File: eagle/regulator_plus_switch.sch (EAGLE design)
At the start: 60 parts, among them IC1 LT1352PA, IC2 LT1352PA, IC3 DG419DJN, IC4 LT1352PA, T1 2N3904, T2 2N3904

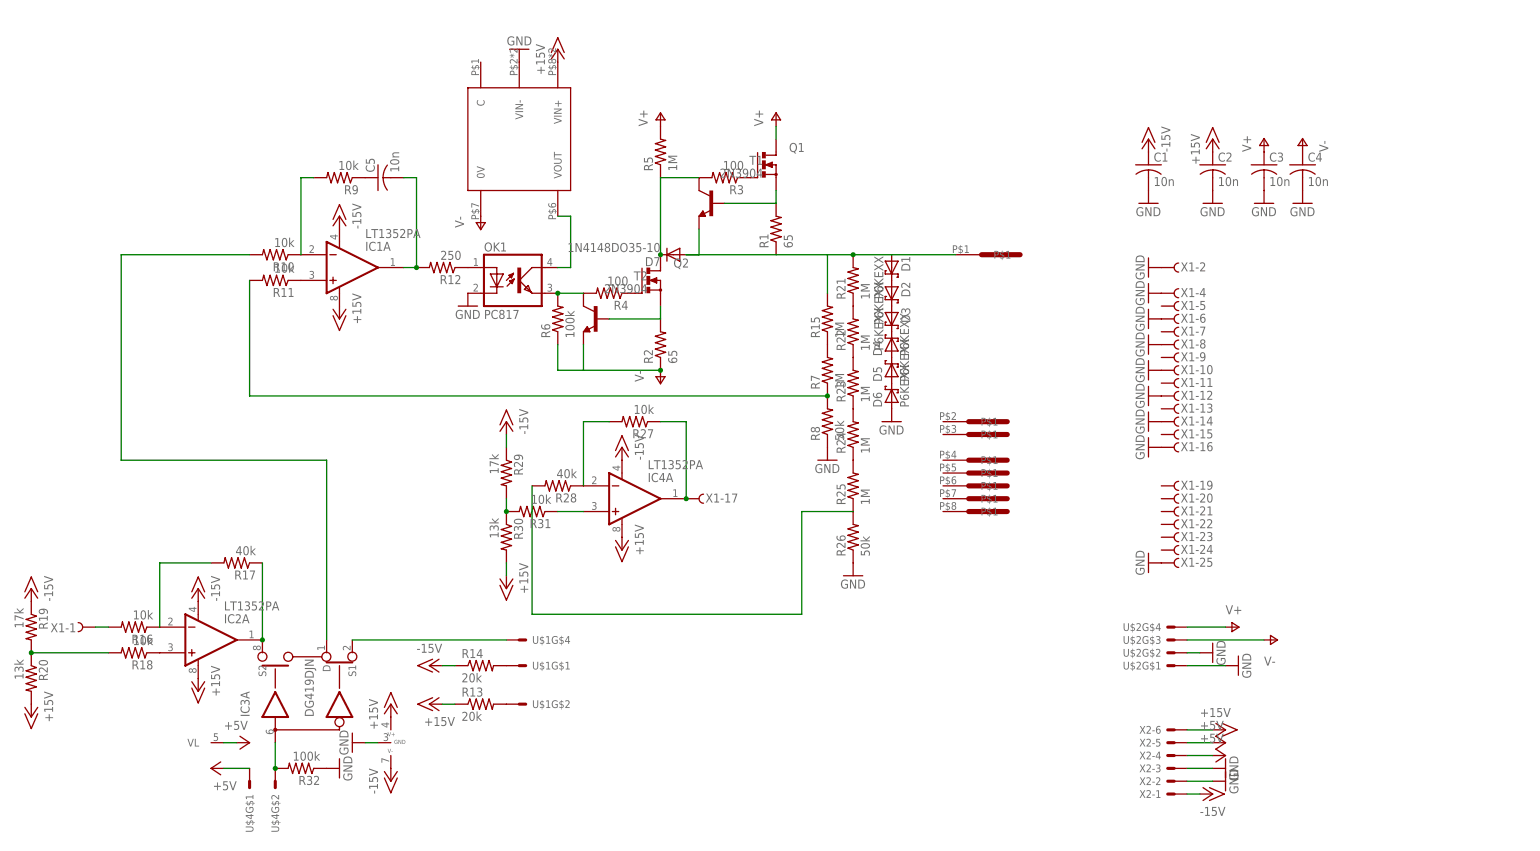
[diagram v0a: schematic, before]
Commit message: pa 97 circuit
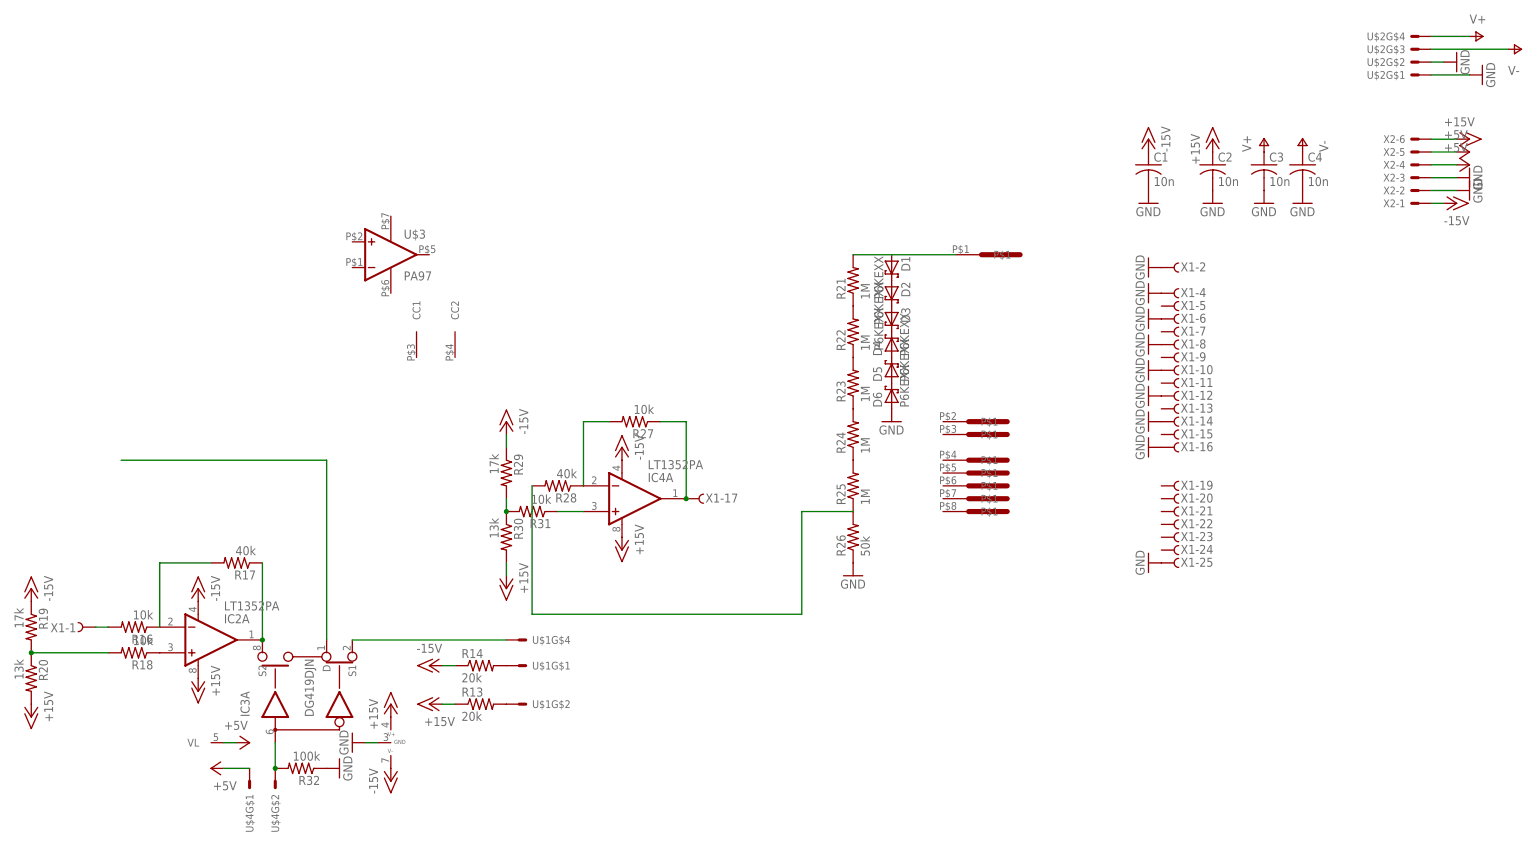
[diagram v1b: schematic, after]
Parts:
- removed C5: 10n, rcl:C-US075-032X103
- removed D7: 1N4148DO35-10, diode:1N4148DO35-10
- removed DC1: (no value), dc-dc-converter:NCS
- removed IC1: LT1352PA, linear-technology:LT1352PA
- removed OK1: PC817, optocoupler:PC817
- removed Q1, Q2: (no value), transistor-power:PMOSFET_NTO220BV
- removed R1, R2: 65, rcl:R-US_0207/10
- removed R10, R11, R9: 10k, rcl:R-US_0207/10
- removed R12: 250, rcl:R-US_0207/15
- removed R15, R5, R7: 1M, resistor:R-US_0414/15
- removed R3, R4: 100, rcl:R-US_0207/10
- removed R6: 100k, rcl:R-US_0207/10
- removed R8: 50k, rcl:R-US_0207/10
- removed T1, T2: 2N3904, transistor:2N3904
- added U$3: PA97, apex:PA97
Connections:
- removed net N$11: Q2.G, R4.1
- removed net N$12: OK1.EMIT, R4.2, R6.2, T2.C
- removed net N$14: Q2.S, R2.2, T2.B
- removed net N$16: DC1.VOUT, OK1.COL
- removed net N$17: C5.1, R9.1
- removed net N$18: IC1A.-IN, R10.1, R9.2
- removed net N$19: C5.2, IC1A.OUT, R12.2
- removed net N$20: IC1A.+IN, R11.1
- removed net N$21: R11.2, R7.1, R8.2
- removed net N$22: OK1.A, R12.1
- removed net N$23: R15.1, R7.2
- removed net N$6: Q1.G, R3.1
- removed net N$7: D7.C, Q2.D, R3.2, R5.1, T1.C
- removed net N$8: Q1.S, R1.2, T1.B
- net +15V: no longer DC1.VIN+, IC1A.V+
- net -15V: no longer IC1A.V-
- net GND: no longer DC1.VIN-, OK1.C, R8.1
- net N$10: no longer D7.A, R1.1, R15.2, T1.E
- net N$28: no longer R10.2
- net V+: no longer Q1.D, R5.2
- net V-: no longer DC1.0V, R2.1, R6.1, T2.E
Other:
- moved on the sheet: U$2G$1, U$2G$2, U$2G$3, U$2G$4, X2-1, X2-2, X2-3, X2-4, X2-5, X2-6
